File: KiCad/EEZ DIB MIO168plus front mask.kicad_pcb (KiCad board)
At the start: 2 copper layers, 17.6 x 111.5 mm, 3 parts

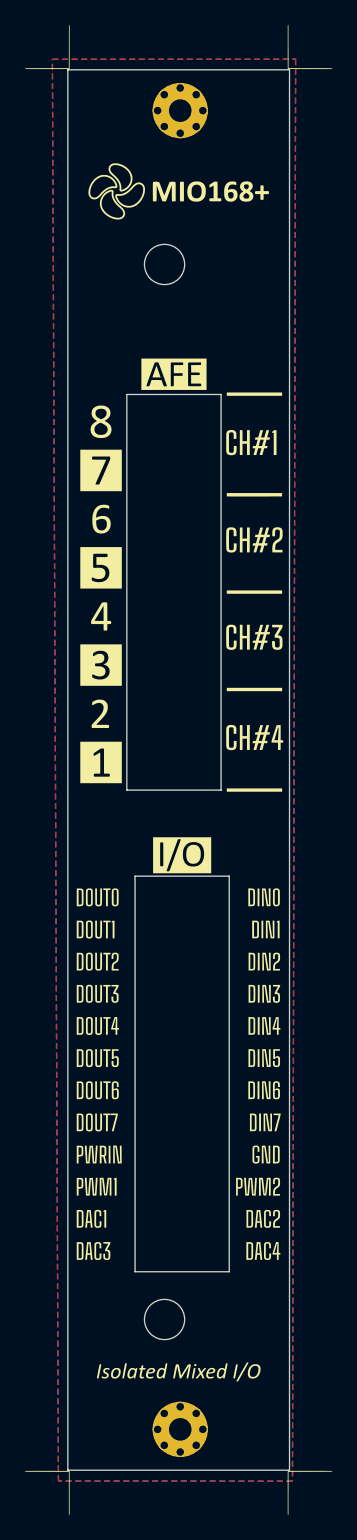
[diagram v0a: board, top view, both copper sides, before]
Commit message: #4
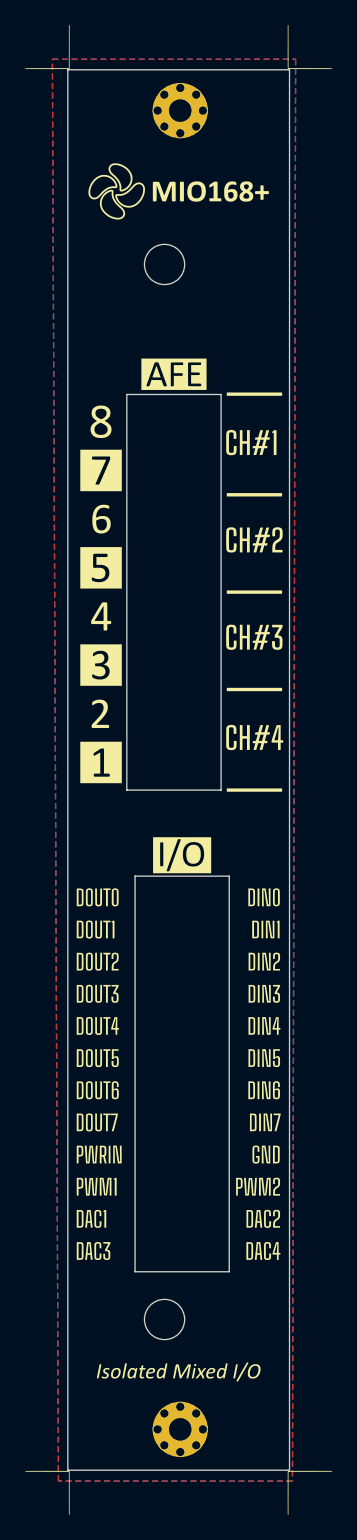
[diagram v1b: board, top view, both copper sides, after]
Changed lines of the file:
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@@
 		(capping no)
 		(filling no)
-		(zone_defaults)
 		(pcbplotparams
 			(layerselection 0x00000000_00000000_55555555_57557573)
@@
 			(at -1.8 0)
 			(size 0.8 0.8)
-			(drill 0.6)
+			(drill 0.65)
 			(layers "*.Cu" "F.Mask")
 			(remove_unused_layers no)
@@
 			(at -1.27 -1.27)
 			(size 0.8 0.8)
-			(drill 0.6)
+			(drill 0.65)
 			(layers "*.Cu" "F.Mask")
 			(remove_unused_layers no)
@@
 			(at -1.27 1.27)
 			(size 0.8 0.8)
-			(drill 0.6)
+			(drill 0.65)
 			(layers "*.Cu" "F.Mask")
 			(remove_unused_layers no)
@@
 			(at 0 -1.8)
 			(size 0.8 0.8)
-			(drill 0.6)
+			(drill 0.65)
 			(layers "*.Cu" "F.Mask")
 			(remove_unused_layers no)
@@
 			(at 0 1.8)
 			(size 0.8 0.8)
-			(drill 0.6)
+			(drill 0.65)
 			(layers "*.Cu" "F.Mask")
 			(remove_unused_layers no)
@@
 			(at 1.27 -1.27)
 			(size 0.8 0.8)
-			(drill 0.6)
+			(drill 0.65)
 			(layers "*.Cu" "F.Mask")
 			(remove_unused_layers no)
@@
 			(at 1.27 1.27)
 			(size 0.8 0.8)
-			(drill 0.6)
+			(drill 0.65)
 			(layers "*.Cu" "F.Mask")
 			(remove_unused_layers no)
@@
 			(at 1.8 0)
 			(size 0.8 0.8)
-			(drill 0.6)
+			(drill 0.65)
 			(layers "*.Cu" "F.Mask")
 			(remove_unused_layers no)
@@
 			(at -1.8 0)
 			(size 0.8 0.8)
-			(drill 0.6)
+			(drill 0.65)
 			(layers "*.Cu" "F.Mask")
 			(remove_unused_layers no)
@@
 			(at -1.27 -1.27)
 			(size 0.8 0.8)
-			(drill 0.6)
+			(drill 0.65)
 			(layers "*.Cu" "F.Mask")
 			(remove_unused_layers no)
@@
 			(at -1.27 1.27)
 			(size 0.8 0.8)
-			(drill 0.6)
+			(drill 0.65)
 			(layers "*.Cu" "F.Mask")
 			(remove_unused_layers no)
@@
 			(at 0 -1.8)
 			(size 0.8 0.8)
-			(drill 0.6)
+			(drill 0.65)
 			(layers "*.Cu" "F.Mask")
 			(remove_unused_layers no)
@@
 			(at 0 1.8)
 			(size 0.8 0.8)
-			(drill 0.6)
+			(drill 0.65)
 			(layers "*.Cu" "F.Mask")
 			(remove_unused_layers no)
@@
 			(at 1.27 -1.27)
 			(size 0.8 0.8)
-			(drill 0.6)
+			(drill 0.65)
 			(layers "*.Cu" "F.Mask")
 			(remove_unused_layers no)
@@
 			(at 1.27 1.27)
 			(size 0.8 0.8)
-			(drill 0.6)
+			(drill 0.65)
 			(layers "*.Cu" "F.Mask")
 			(remove_unused_layers no)
@@
 			(at 1.8 0)
 			(size 0.8 0.8)
-			(drill 0.6)
-			(layers "*.Cu" "F.Mask")
-			(remove_unused_layers no)
+			(drill 0.65)
+			(layers "*.Cu" "F.Mask")
+			(remove_unused_layers no)
